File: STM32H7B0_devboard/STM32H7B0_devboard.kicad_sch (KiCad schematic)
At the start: 85 parts, among them J1 SWD, J2 24LC512 socet, J4 PORT_A, J5 PORT_B, J6 PORT_C, J7 PORT_D, J8 PORT_E, J9 Power_Conn, Q1 S8050, U1 STM32H7B0VBT6, Y1 32.768KHz, Y2 25MHz

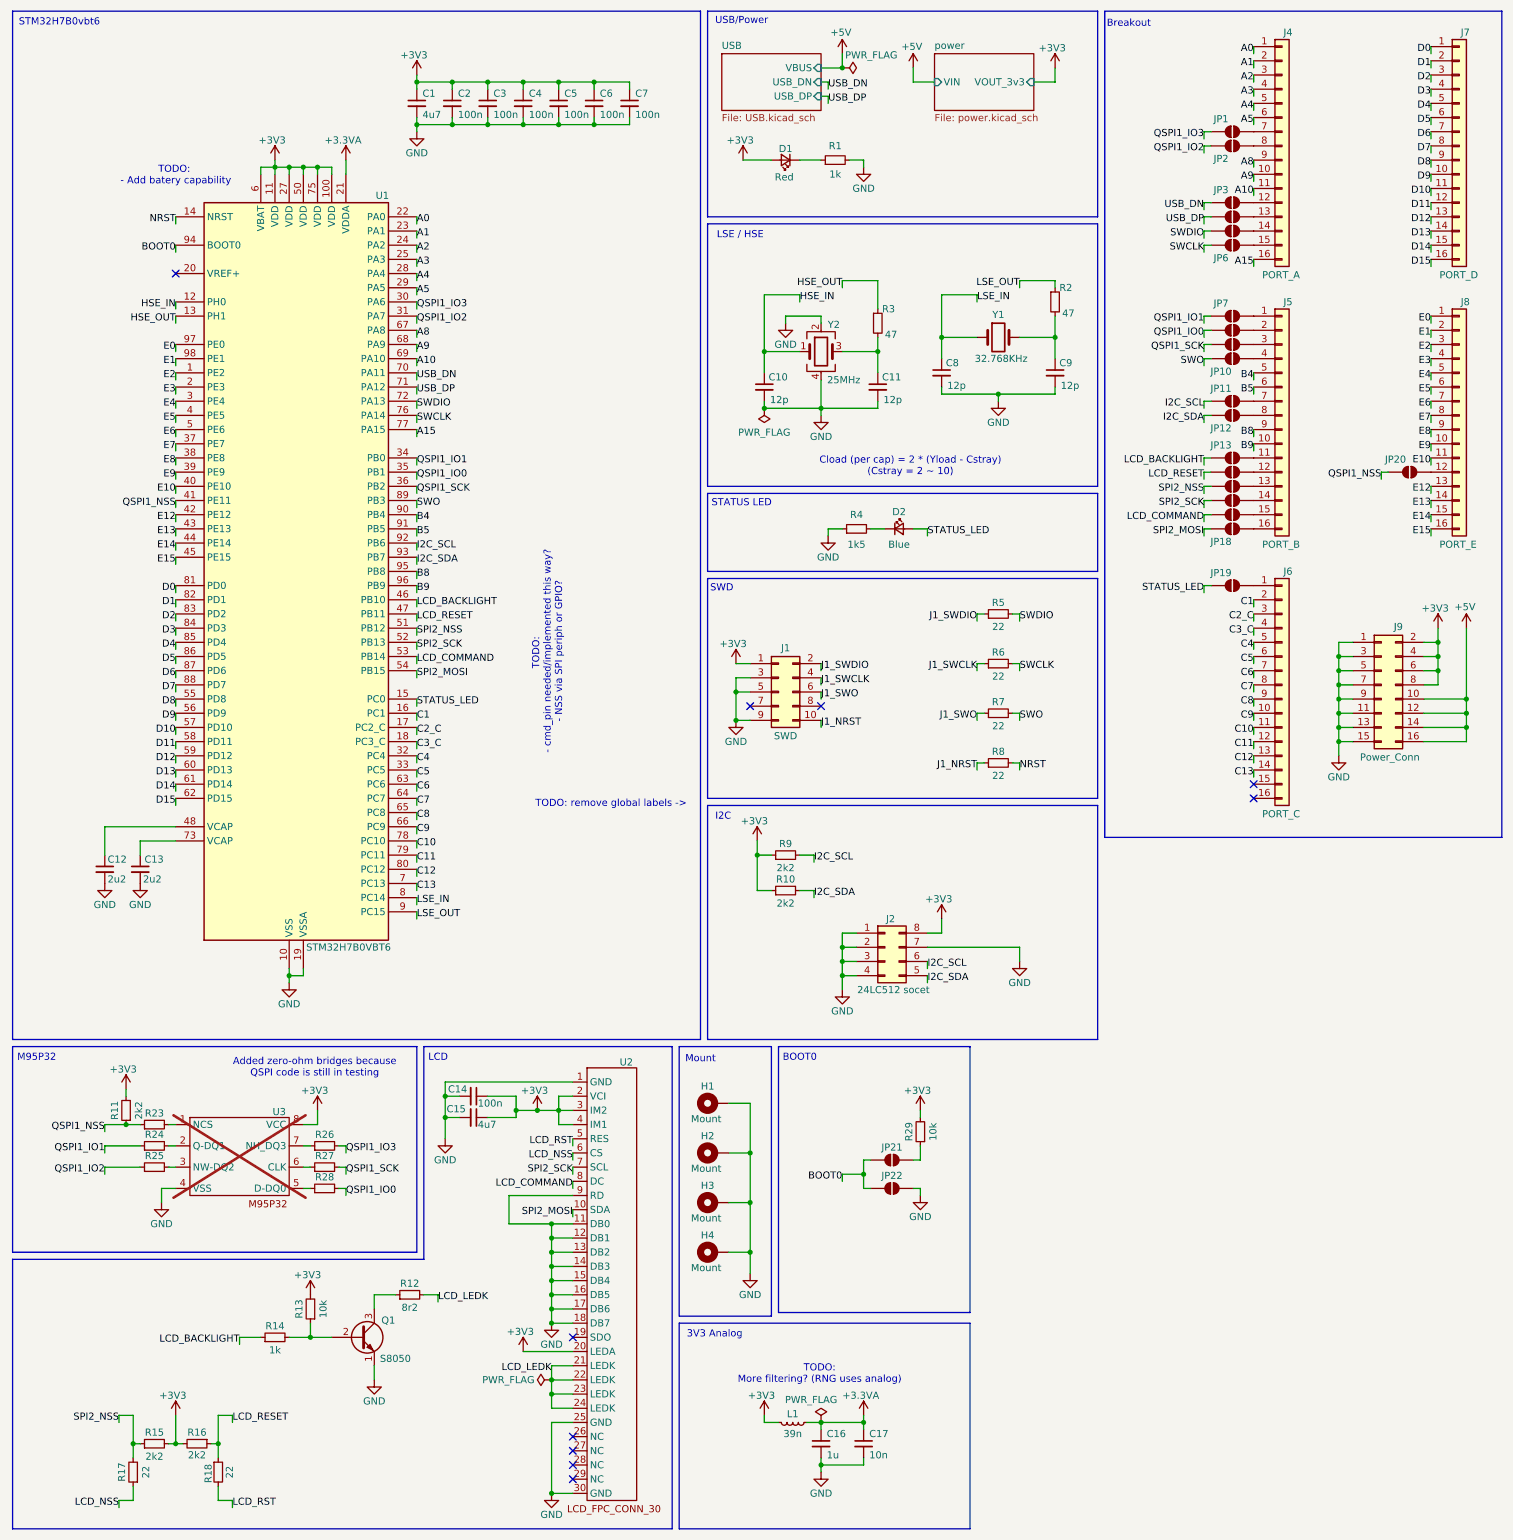
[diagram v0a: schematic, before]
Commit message: Started on V2
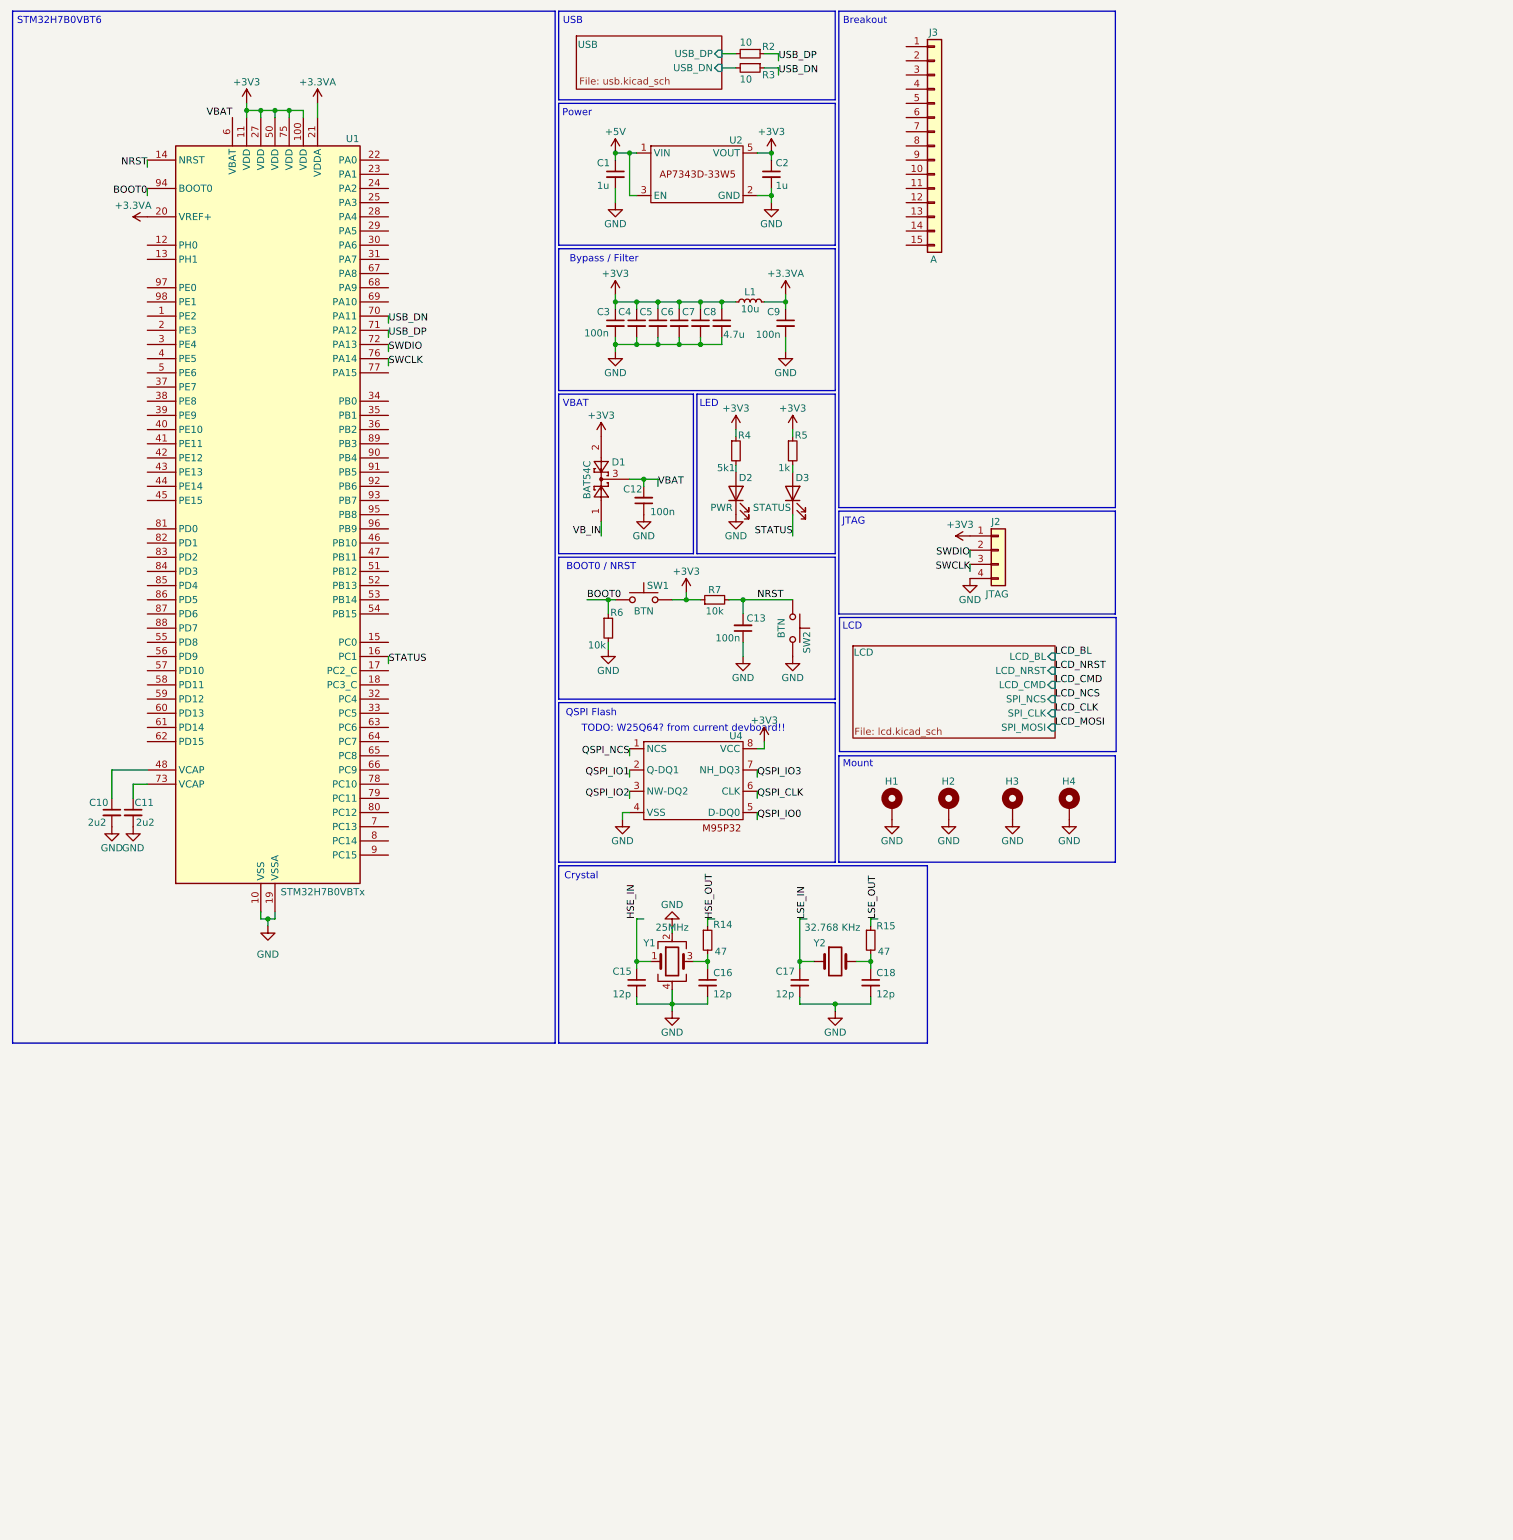
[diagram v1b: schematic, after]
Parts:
- removed C14: 100n, Capacitor_SMD:C_0402_1005Metric, symbol Device:C_Small
- removed D1: Red, Diode_SMD:D_0603_1608Metric, symbol Device:LED_Small
- removed D2: Blue, Diode_SMD:D_0603_1608Metric, symbol Device:LED_Small
- removed J1: SWD, Connector_PinSocket_2.00mm:PinSocket_2x05_P2.00mm_Vertical, symbol Connector_Generic:Conn_02x05_Odd_Even
- removed J2: 24LC512 socet, Package_DIP:CERDIP-8_W7.62mm_SideBrazed_Socket, symbol Connector_Generic:Conn_02x04_Counter_Clockwise
- removed J4: PORT_A, Connector_PinSocket_2.00mm:PinSocket_1x16_P2.00mm_Vertical, symbol Connector_Generic:Conn_01x16
- removed J5: PORT_B, Connector_PinSocket_2.00mm:PinSocket_1x16_P2.00mm_Vertical, symbol Connector_Generic:Conn_01x16
- removed J6: PORT_C, Connector_PinSocket_2.00mm:PinSocket_1x16_P2.00mm_Vertical, symbol Connector_Generic:Conn_01x16
- removed J7: PORT_D, Connector_PinSocket_2.00mm:PinSocket_1x16_P2.00mm_Vertical, symbol Connector_Generic:Conn_01x16
- removed J8: PORT_E, Connector_PinSocket_2.00mm:PinSocket_1x16_P2.00mm_Vertical, symbol Connector_Generic:Conn_01x16
- removed J9: Power_Conn, Connector_PinSocket_2.00mm:PinSocket_2x08_P2.00mm_Vertical, symbol Connector_Generic:Conn_02x08_Odd_Even
- removed JP1, JP10, JP11, JP12, JP13, JP14, JP15, JP16, JP17, JP18, JP19, JP2, JP20, JP21, JP22, JP3, JP4, JP5, JP6, JP7, JP8, JP9: ~, Jumper:SolderJumper-2_P1.3mm_Open_TrianglePad1.0x1.5mm, symbol Jumper:SolderJumper_2_Open
- removed Q1: S8050, Package_TO_SOT_SMD:SOT-23, symbol Transistor_BJT:S8050
- removed R1: 1k, Resistor_SMD:R_0603_1608Metric, symbol Device:R_Small
- removed R10, R11, R16, R9: 2k2, Resistor_SMD:R_0402_1005Metric, symbol Device:R_Small
- removed R12: 8r2, Resistor_SMD:R_0402_1005Metric, symbol Device:R_Small
- removed R13, R29: 10k, Resistor_SMD:R_0402_1005Metric, symbol Device:R_Small
- removed R17, R18, R8: 22, Resistor_SMD:R_0402_1005Metric, symbol Device:R_Small
- removed R23, R24, R25, R26, R27, R28: 0, Resistor_SMD:R_0603_1608Metric, symbol Device:R_Small
- removed U2: ~, Custom:FPC_30_soldered, symbol Marijn:1.9{dblquote} LCD_FPC_CONN
- removed U3: ~, Package_SO:PowerIntegrations_SO-8, symbol Marijn:M95P32
- removed Y1: 32.768KHz, Crystal:Crystal_SMD_3215-2Pin_3.2x1.5mm, symbol Device:Crystal
- removed Y2: 25MHz, Crystal:Crystal_SMD_3225-4Pin_3.2x2.5mm, symbol Device:Crystal_GND24
- added C18: 12p, Capacitor_SMD:C_0402_1005Metric, symbol Device:C_Small
- added D1: BAT54C, Package_TO_SOT_SMD:SOT-23, symbol Diode:BAT54C
- added D2: PWR, symbol Device:LED
- added D3: STATUS, symbol Device:LED
- added J2: JTAG, symbol Connector_Generic:Conn_01x04
- added J3: A, symbol Connector_Generic:Conn_01x15
- added SW1, SW2: BTN, symbol Switch:SW_Push
- added U2: ~, Custom:SOT-25, symbol Marijn:AP7343
- added U4: ~, symbol Marijn:M95P32
- added Y1: 25MHz, Crystal:Crystal_SMD_3225-4Pin_3.2x2.5mm, symbol Device:Crystal_GND24
- added Y2: 32.768 KHz, Crystal:Crystal_SMD_3215-2Pin_3.2x1.5mm, symbol Device:Crystal
- C1: value 4u7 -> 1u; footprint Capacitor_SMD:C_0402_1005Metric -> (none); LCSC C23733 -> (none)
- C10, C11: value 12p -> 2u2; LCSC C1547 -> C12530
- C12, C13: value 2u2 -> 100n; footprint Capacitor_SMD:C_0402_1005Metric -> (none); LCSC C12530 -> (none)
- C15: value 4u7 -> 12p; LCSC C23733 -> C1547
- C16: value 1u -> 12p; LCSC C52923 -> C1547
- C17: value 10n -> 12p; LCSC C15195 -> C1547
- C2: value 100n -> 1u; footprint Capacitor_SMD:C_0402_1005Metric -> (none); LCSC C1525 -> (none)
- C3, C4, C5, C6, C7: footprint Capacitor_SMD:C_0402_1005Metric -> (none); LCSC C1525 -> (none)
- C8: value 12p -> 4.7u; footprint Capacitor_SMD:C_0402_1005Metric -> (none); LCSC C1547 -> (none)
- C9: value 12p -> 100n; footprint Capacitor_SMD:C_0402_1005Metric -> (none); LCSC C1547 -> (none)
- H1, H2, H3, H4: value Mount -> MountingHole_Pad; footprint MountingHole:MountingHole_4.3mm_M4_Pad_Via -> (none)
- L1: value 39n -> 10u; footprint Inductor_SMD:L_0603_1608Metric -> (none); LCSC C74308 -> (none)
- R14: value 1k -> 47; LCSC C11702 -> C25118
- R15: value 2k2 -> 47; LCSC C25879 -> C25118
- R2, R3: value 47 -> 10; footprint Resistor_SMD:R_0402_1005Metric -> (none); LCSC C25118 -> (none)
- R4: value 1k5 -> 5k1; footprint Resistor_SMD:R_0603_1608Metric -> (none); LCSC C22843 -> (none)
- R5: value 22 -> 1k; footprint Resistor_SMD:R_0402_1005Metric -> (none); LCSC C25092 -> (none)
- R6, R7: value 22 -> 10k; footprint Resistor_SMD:R_0402_1005Metric -> (none); LCSC C25092 -> (none)
- U1: value STM32H7B0VBT6 -> STM32H7B0VBTx; LCSC C730227 -> (none)
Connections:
- net J1_SWCLK is gone; now on net BOOT0: R6.1
- net J1_SWDIO is gone; now on net +3V3: R5.1
- net J1_SWO is gone; now on net +3V3: R7.1
- net +3.3VA: now also C9.1, L1.2, U1.20 (VREF+); no longer C16.1, C17.1, L1.1
- net +3V3: now also C8.1, L1.1, R4.1, D1.2, J2.1 (Pin_1), SW1.2, U2.5 (VOUT), U4.8 (VCC); no longer C1.1, C15.1, L1.2, R15.2, U1.6 (VBAT)
- net +5V: now also C1.1, U2.1 (VIN), U2.3 (EN)
- net BOOT0: now also SW1.1
- net GND: now also C12.1, C13.1, R6.2, C18.2, D2.1 (K), J2.4 (Pin_4), SW2.2, U2.2 (GND), U4.4 (VSS), Y1.2, Y1.4; no longer C12.2, C13.2, R4.1
- net HSE_IN: now also C15.1, Y1.1; no longer C10.1, U1.12 (PH0)
- net HSE_OUT: now also R14.1; no longer R3.1, U1.13 (PH1)
- net LSE_IN: now also C17.1, Y2.1; no longer C8.1, U1.8 (PC14)
- net LSE_OUT: now also R15.1; no longer R2.1, U1.9 (PC15)
- net NRST: now also C13.2, R7.2, SW2.1
- net SWCLK: now also J2.3 (Pin_3); no longer R6.2
- net SWDIO: now also J2.2 (Pin_2); no longer R5.2
- net USB_DN: now also R3.1
- net USB_DP: now also R2.1
- net USB/USB_DP: now reaches R2.2
- net USB/USB_DP: no longer C9.1
- net at R14.2: now also C16.1, Y1.3
- net at C11.1: now also U1.73 (VCAP); no longer R3.2
- net at U1.48 (VCAP): now also C10.1; no longer C12.1
- net at R4.2: now also D2.2 (A)
- net A0: no longer names the net of U1.22 (PA0)
- net A1: no longer names the net of U1.23 (PA1)
- net A10: no longer names the net of U1.69 (PA10)
- net A15: no longer names the net of U1.77 (PA15)
- net A2: no longer names the net of U1.24 (PA2)
- net A3: no longer names the net of U1.25 (PA3)
- net A4: no longer names the net of U1.28 (PA4)
- net A5: no longer names the net of U1.29 (PA5)
- net A8: no longer names the net of U1.67 (PA8)
- net A9: no longer names the net of U1.68 (PA9)
- net B4: no longer names the net of U1.90 (PB4)
- net B5: no longer names the net of U1.91 (PB5)
- net B8: no longer names the net of U1.95 (PB8)
- net B9: no longer names the net of U1.96 (PB9)
- net C1 renamed STATUS
- net STATUS: now also D3.1 (K)
- net C10: no longer names the net of U1.78 (PC10)
- net C11: no longer names the net of U1.79 (PC11)
- net C12: no longer names the net of U1.80 (PC12)
- net C13: no longer names the net of U1.7 (PC13)
- net C2_C: no longer names the net of U1.17 (PC2_C)
- net C3_C: no longer names the net of U1.18 (PC3_C)
- net C4: no longer names the net of U1.32 (PC4)
- net C5: no longer names the net of U1.33 (PC5)
- net C6: no longer names the net of U1.63 (PC6)
- net C7: no longer names the net of U1.64 (PC7)
- net C8: no longer names the net of U1.65 (PC8)
- net C9: no longer names the net of U1.66 (PC9)
- net D0: no longer names the net of U1.81 (PD0)
- net D1: no longer names the net of U1.82 (PD1)
- net D10: no longer names the net of U1.57 (PD10)
- net D11: no longer names the net of U1.58 (PD11)
- net D12: no longer names the net of U1.59 (PD12)
- net D13: no longer names the net of U1.60 (PD13)
- net D14: no longer names the net of U1.61 (PD14)
- net D15: no longer names the net of U1.62 (PD15)
- net D2: no longer names the net of U1.83 (PD2)
- net D3: no longer names the net of U1.84 (PD3)
- net D4: no longer names the net of U1.85 (PD4)
- net D5: no longer names the net of U1.86 (PD5)
- net D6: no longer names the net of U1.87 (PD6)
- net D7: no longer names the net of U1.88 (PD7)
- net D8: no longer names the net of U1.55 (PD8)
- net D9: no longer names the net of U1.56 (PD9)
- net E0: no longer names the net of U1.97 (PE0)
- net E1: no longer names the net of U1.98 (PE1)
- net E10: no longer names the net of U1.40 (PE10)
- net E12: no longer names the net of U1.42 (PE12)
- net E13: no longer names the net of U1.43 (PE13)
- net E14: no longer names the net of U1.44 (PE14)
- net E15: no longer names the net of U1.45 (PE15)
- net E2: no longer names the net of U1.1 (PE2)
- net E3: no longer names the net of U1.2 (PE3)
- net E4: no longer names the net of U1.3 (PE4)
- net E5: no longer names the net of U1.4 (PE5)
- net E6: no longer names the net of U1.5 (PE6)
- net E7: no longer names the net of U1.37 (PE7)
- net E8: no longer names the net of U1.38 (PE8)
- net E9: no longer names the net of U1.39 (PE9)
- net I2C_SCL: no longer names the net of U1.92 (PB6)
- net I2C_SDA: no longer names the net of U1.93 (PB7)
- net LCD_BACKLIGHT: no longer names the net of U1.46 (PB10)
- net LCD_BACKLIGHT: no longer R14.1
- net LCD_COMMAND: no longer names the net of U1.53 (PB14)
- net LCD_RESET: no longer names the net of U1.47 (PB11)
- net QSPI1_IO0: no longer names the net of U1.35 (PB1)
- net QSPI1_IO1: no longer names the net of U1.34 (PB0)
- net QSPI1_IO2: no longer names the net of U1.31 (PA7)
- net QSPI1_IO3: no longer names the net of U1.30 (PA6)
- net QSPI1_NSS: no longer names the net of U1.41 (PE11)
- net QSPI1_SCK: no longer names the net of U1.36 (PB2)
- net SPI2_MOSI: no longer names the net of U1.54 (PB15)
- net SPI2_NSS: no longer names the net of U1.51 (PB12)
- net SPI2_NSS: no longer R15.1
- net SPI2_SCK: no longer names the net of U1.52 (PB13)
- net STATUS_LED: no longer names the net of U1.15 (PC0)
- net SWO: no longer names the net of U1.89 (PB3)
- net SWO: no longer R7.2
- new net: C18.1, R15.2, Y2.2
- new net: D3.2 (A), R5.2
- new net QSPI_CLK: U4.6 (CLK)
- new net QSPI_IO0: U4.5 (D-DQ0)
- new net QSPI_IO1: U4.2 (Q-DQ1)
- new net QSPI_IO2: U4.3 (NW-DQ2)
- new net QSPI_IO3: U4.7 (NH_DQ3)
- new net QSPI_NCS: U4.1 (NCS)
- new net USB/USB_DN: R3.2
- new net VBAT: C12.2, D1.3, U1.6 (VBAT)
- new net VB_IN: D1.1
- no-connect marks 10 -> 0
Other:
- removed sheet power
- added sheet LCD (lcd.kicad_sch)
- sheet USB: file USB.kicad_sch -> usb.kicad_sch
- sheet USB ports: added none; removed VBUS
- note added: "BOOT0 / NRST"
- note added: "Bypass / Filter"
- note added: "Crystal"
- note added: "JTAG"
- note added: "LED"
- note added: "Power"
- note added: "QSPI Flash"
- note added: "STM32H7B0VBT6"
- note added: "TODO: W25Q64? from current devboard!!"
- note added: "USB"
- note added: "VBAT"
- note removed: "3V3 Analog"
- note removed: "Added zero-ohm bridges because QSPI code is still in testing"
- note removed: "BOOT0"
- note removed: "Cload (per cap) = 2 * (Yload - Cstray) (Cstray = 2 ~ 10)"
- note removed: "I2C"
- note removed: "LSE / HSE"
- note removed: "M95P32"
- note removed: "STATUS LED"
- note removed: "STM32H7B0vbt6"
- note removed: "SWD"
- note removed: "TODO: - Add batery capability"
- note removed: "TODO: - cmd_pin needed/implemented this way? - NSS via SPI periph or GPIO?"
- note removed: "TODO: More filtering? (RNG uses analog)"
- note removed: "TODO: remove global labels ->"
- note removed: "USB/Power"
- company: Marijn Verschuren -> (none)
- title: STM32H7B0_devboard -> (none)
